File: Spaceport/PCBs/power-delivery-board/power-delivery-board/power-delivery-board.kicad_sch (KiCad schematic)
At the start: 26 parts, among them J1 Conn_01x03_Pin, U1 ADP5033ACBZ-5-R7, U2 TPS610986DSER, U3 TPS610986DSER

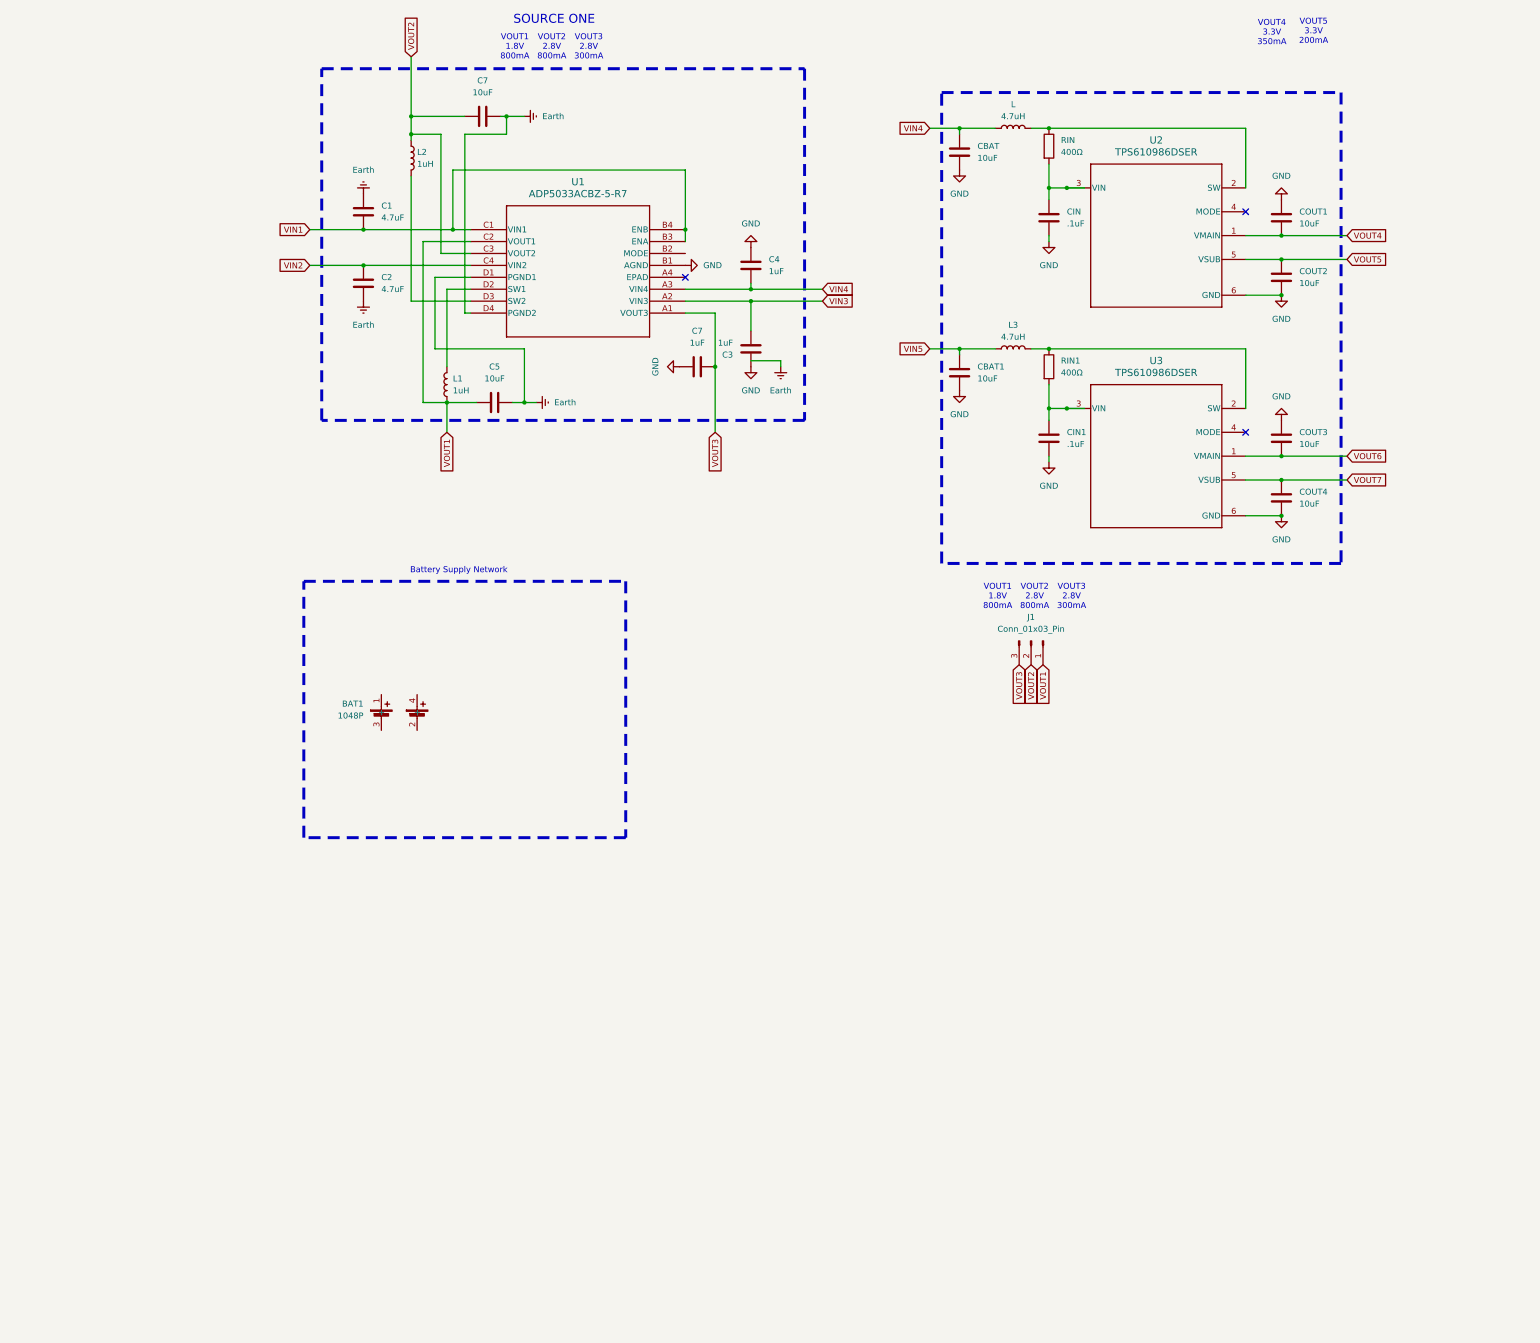
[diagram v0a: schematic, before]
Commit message: Updated JST Pin
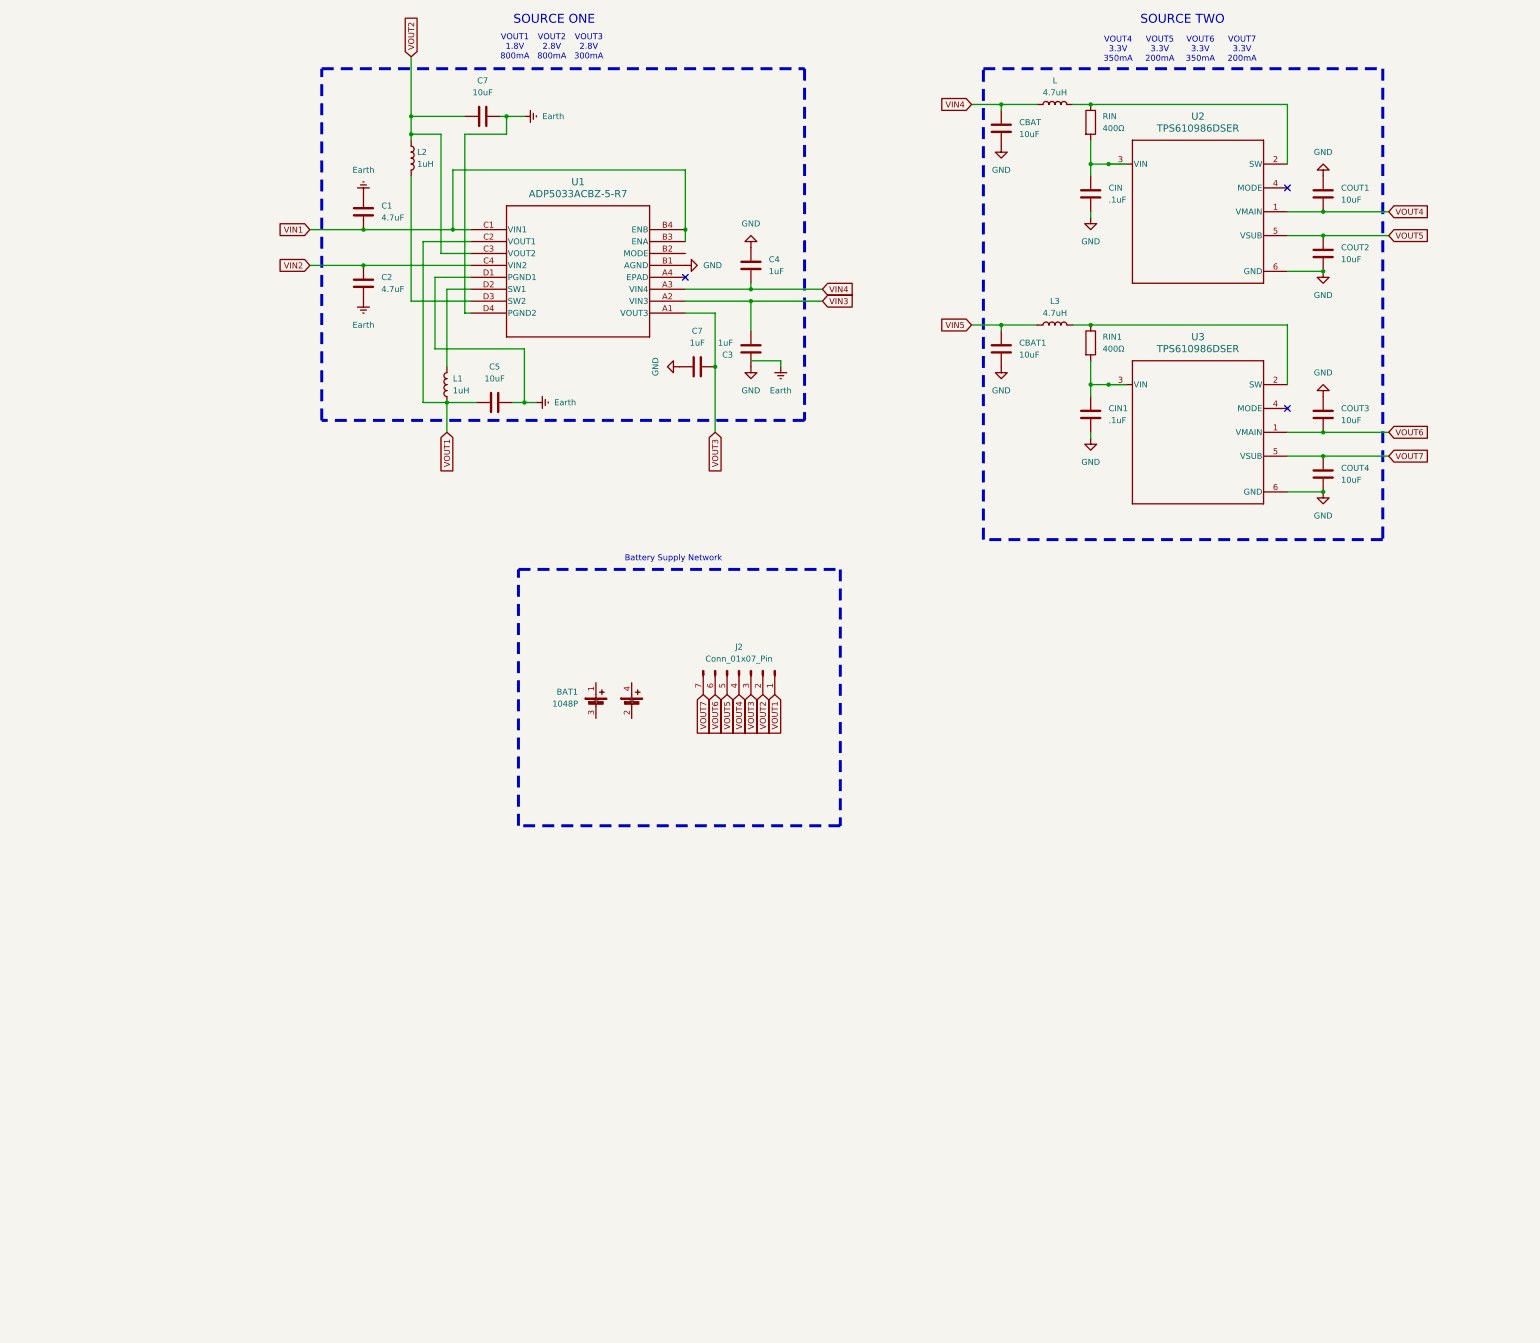
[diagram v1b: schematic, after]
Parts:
- removed J1: Conn_01x03_Pin, symbol Connector:Conn_01x03_Pin
- added J2: Conn_01x07_Pin, symbol Connector:Conn_01x07_Pin
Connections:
- net VOUT1: now also J2.1 (Pin_1)
- net VOUT2: now also J2.2 (Pin_2)
- net VOUT3: now also J2.3 (Pin_3)
- net VOUT4: now also J2.4 (Pin_4)
- net VOUT5: now also J2.5 (Pin_5)
- net VOUT6: now also J2.6 (Pin_6)
- net VOUT7: now also J2.7 (Pin_7)
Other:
- note added: "SOURCE TWO"
- note added: "VOUT6 3.3V 350mA"
- note added: "VOUT7 3.3V 200mA"
- moved on the sheet: BAT1, CBAT, CBAT1, CIN, CIN1, COUT1, COUT2, COUT3, COUT4, L, L3, RIN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

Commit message: Added LEDS and Labeled VIN
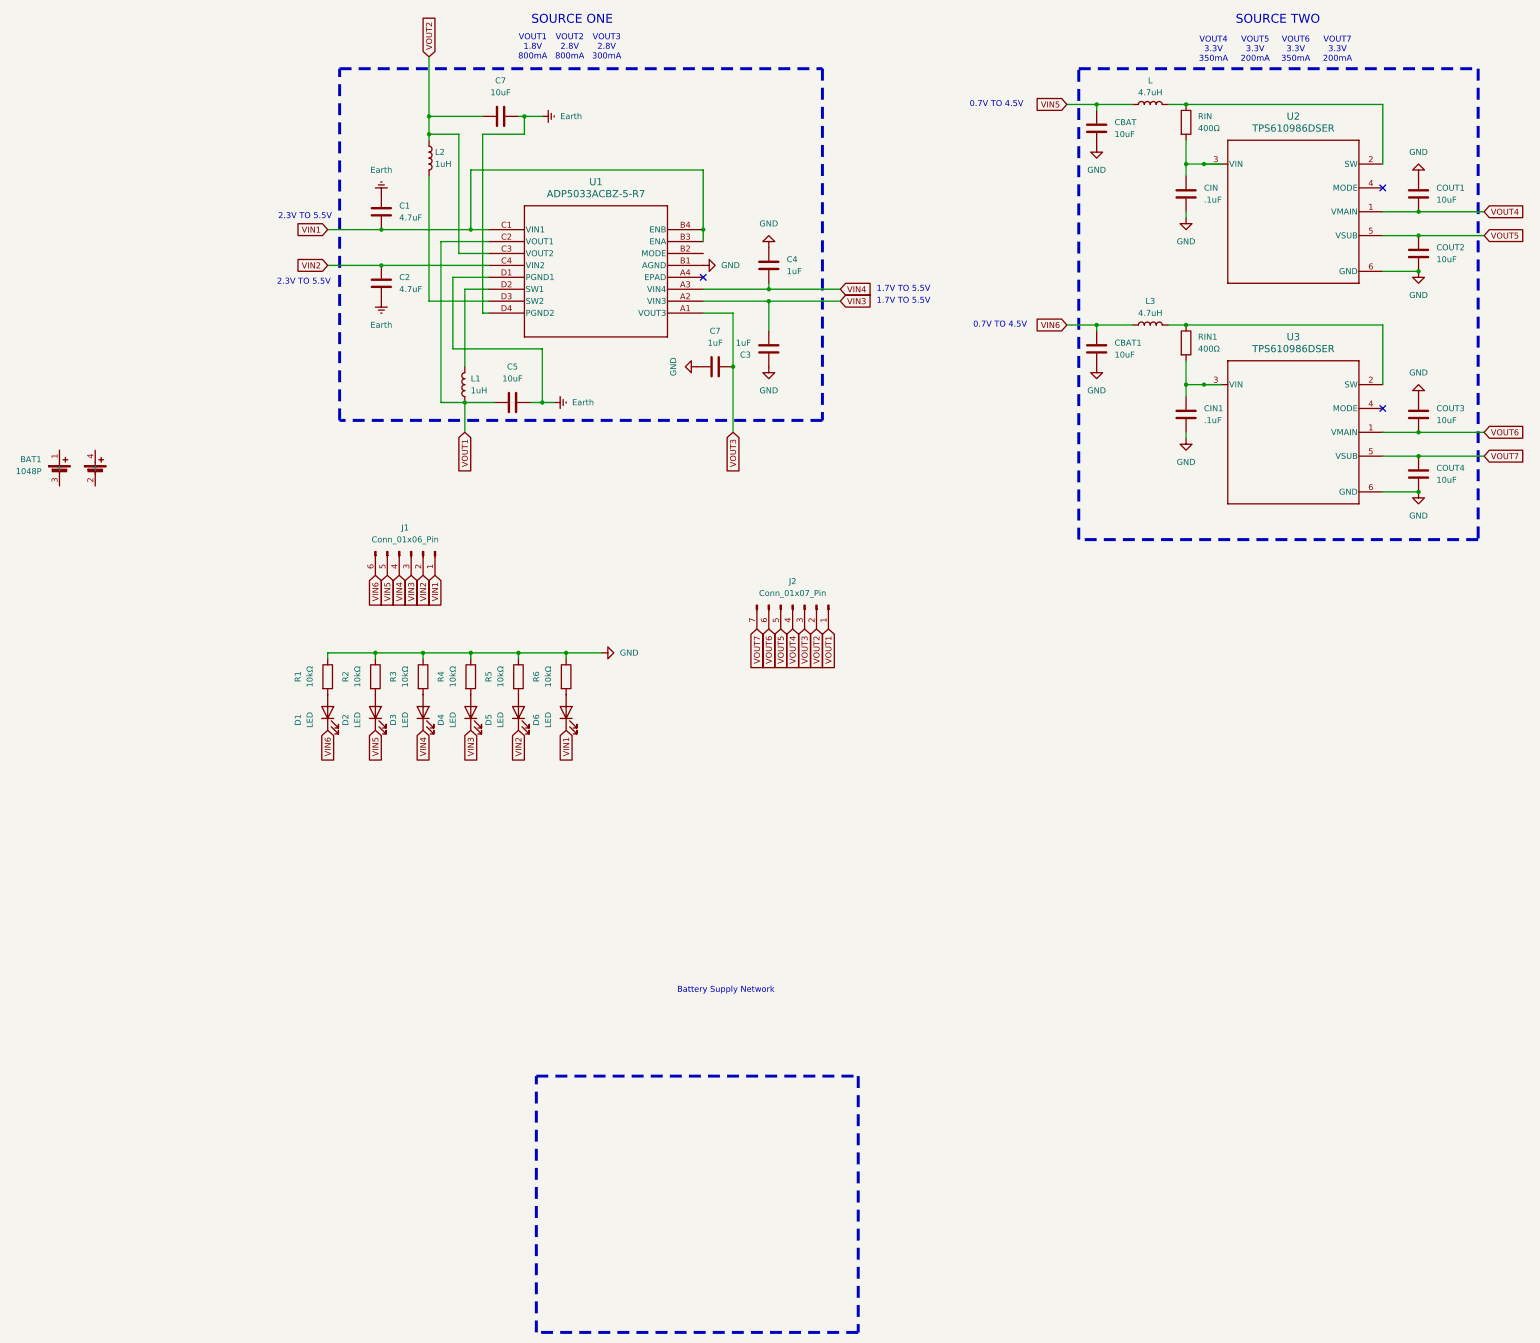
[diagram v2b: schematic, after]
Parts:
- added D1, D2, D3, D4, D5, D6: LED, symbol Device:LED
- added J1: Conn_01x06_Pin, symbol Connector:Conn_01x06_Pin
- added R1, R2, R3, R4, R5, R6: 10kΩ, symbol Device:R
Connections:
- net GND: now also R1.1, R2.1, R3.1, R4.1, R5.1, R6.1
- net VIN1: now also D6.1 (K), J1.1 (Pin_1)
- net VIN2: now also D5.1 (K), J1.2 (Pin_2)
- net VIN3: now also D4.1 (K), J1.3 (Pin_3)
- net VIN4: now also D3.1 (K), J1.4 (Pin_4); no longer CBAT.1, L.1
- net VIN5: now also CBAT.1, L.1, D2.1 (K), J1.5 (Pin_5); no longer CBAT1.1, L3.1
- new net: D1.2 (A), R1.2
- new net: D2.2 (A), R2.2
- new net: D3.2 (A), R3.2
- new net: D6.2 (A), R6.2
- new net: D5.2 (A), R5.2
- new net: D4.2 (A), R4.2
- new net VIN6: CBAT1.1, D1.1 (K), J1.6 (Pin_6), L3.1
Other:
- note added: "0.7V TO 4.5V"
- note added: "1.7V TO 5.5V"
- note added: "2.3V TO 5.5V"
- moved on the sheet: BAT1, C1, C2, C3, C4, C5, C7, CBAT, CBAT1, CIN, CIN1, COUT1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
